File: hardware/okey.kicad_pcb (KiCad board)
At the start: 2 copper layers, 263.4 x 349.9 mm, 160 parts, among them IC1 4094N, IC2 4094N, J1 RJ45, J2 RJ45, P1 ROW_JMP, P10 CONN_02X06, P11 CONN_02X06, P12 CONN_02X06, P13 CONN_02X06, P14 CONN_02X06, P15 CONN_02X06, P16 CONN_02X08, P17 CONN_01X01, P18 CONN_02X08, P19 CONN_01X01, P2 CONN_02X13, P20 CONN_01X01, P21 CONN_01X01, P22 CONN_02X08, P23 CONN_02X08, P24 CONN_02X06, P25 CONN_02X06, P26 CONN_02X06, P27 CONN_02X06, P28 CONN_02X06, P29 CONN_02X06, P3 CONN_02X03, P30 CONN_02X08, P31 CONN_02X03, P32 CONN_02X03, P33 CONN_02X06, P34 CONN_02X06, P35 CONN_02X06, P36 CONN_02X06, P37 CONN_02X06, P38 CONN_02X06, P39 CONN_01X01, P4 CONN_02X08, P40 CONN_02X03, P41 CONN_02X06, P42 CONN_02X06, P43 CONN_02X06, P44 CONN_02X06, P45 CONN_02X06, P46 CONN_02X06, P47 CONN_01X01, P48 CONN_02X03, P5 CONN_02X03, P6 CONN_02X10, P7 CONN_02X03, P8 CONN_01X01, P9 CONN_02X08, Q1 Q_NPN_BCE, Q2 Q_NPN_BCE, Q3 Q_NPN_BCE, SW1 MX_D, SW10 MX_D, SW11 MX_D, SW12 MX_D, SW13 MX_D, SW14 MX_D, SW15 MX_D, SW16 MX_D, SW17 MX_D, SW18 MX_D, SW19 SW_PUSH, SW2 MX_D, SW20 SW_PUSH, SW21 SW_PUSH, SW22 SW_PUSH, SW23 SW_PUSH, SW24 SW_PUSH, SW25 SW_PUSH, SW26 SW_PUSH, SW27 SW_PUSH, SW28 SW_PUSH, SW29 SW_PUSH, SW3 MX_D, SW30 SW_PUSH, SW31 SW_PUSH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

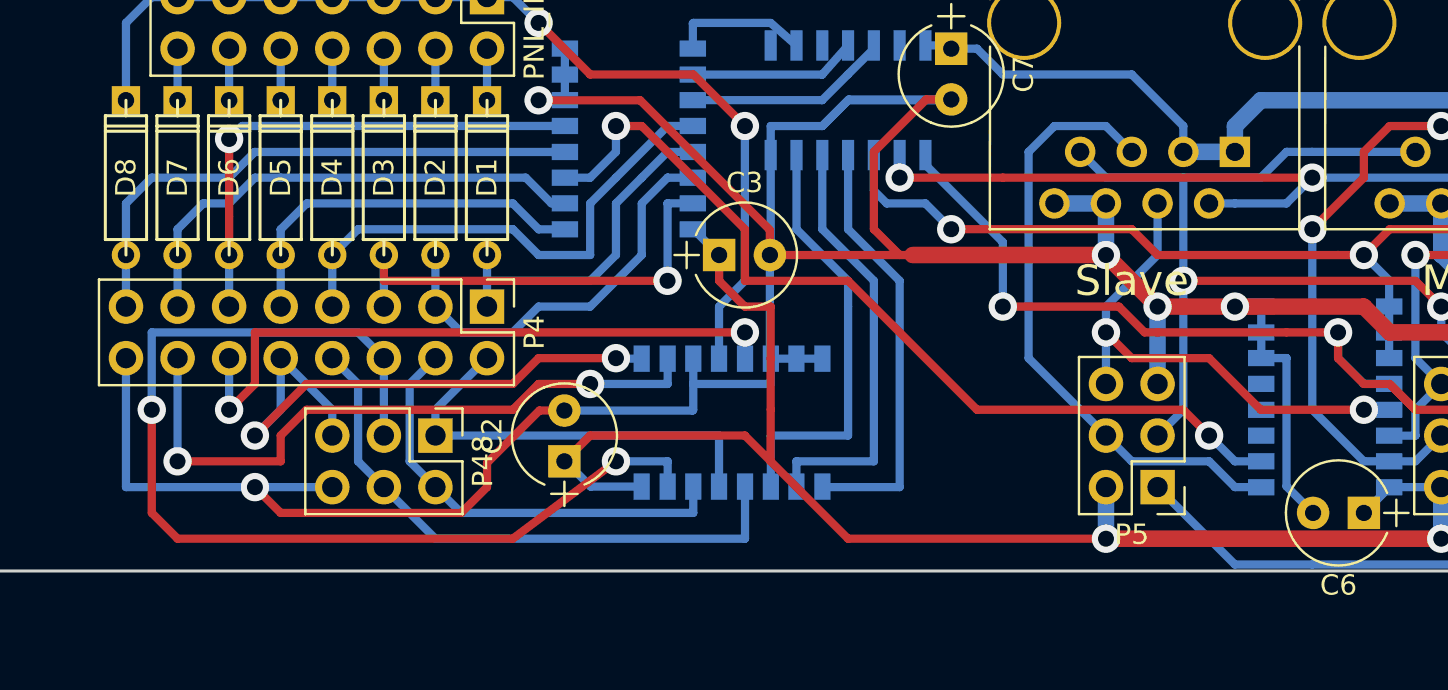
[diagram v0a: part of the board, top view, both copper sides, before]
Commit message: ...
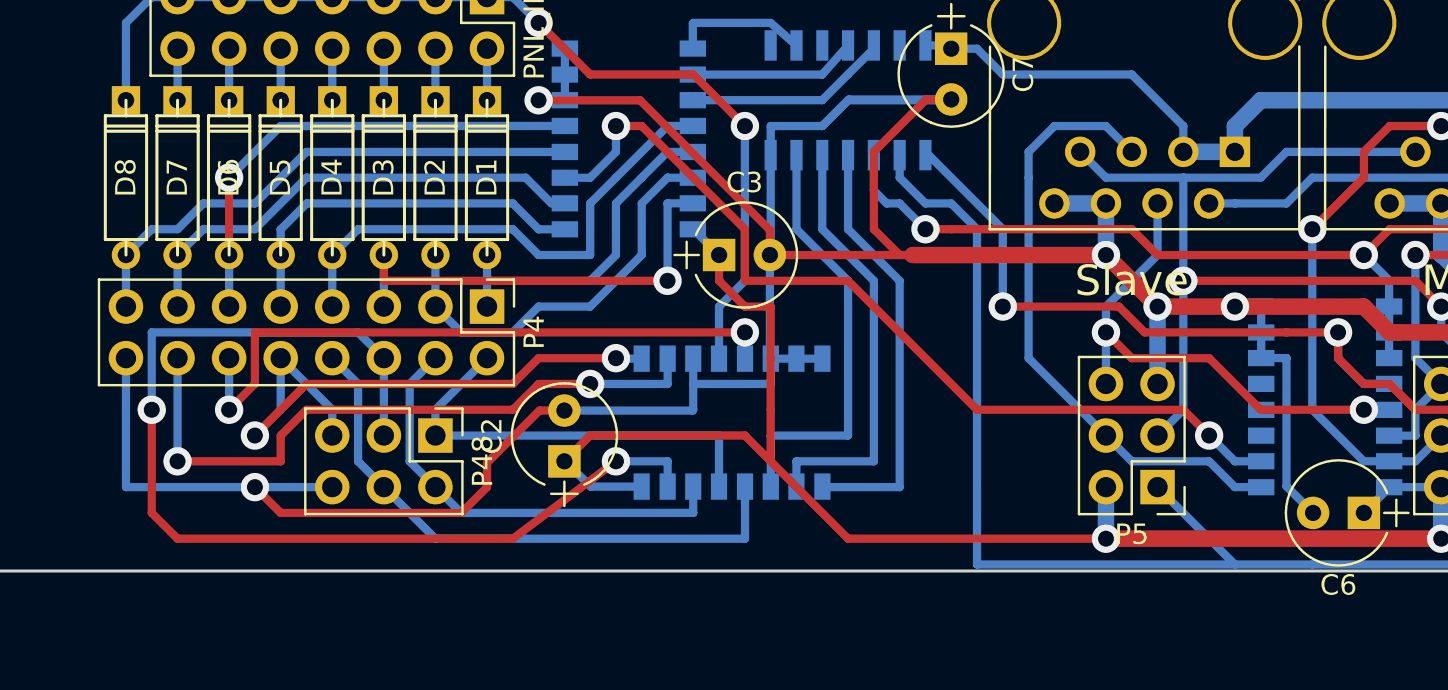
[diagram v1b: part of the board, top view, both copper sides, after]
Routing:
- net /Panel Generic SPI01/reset: track 85.6 -> 99.4 mm, vias 2 -> 0
- net Net-(D8-Pad2): track 27.7 -> 26.3 mm
- net Net-(D6-Pad2): track 25.1 -> 23.9 mm
- net Net-(D7-Pad2): track 24.5 -> 23.7 mm
- net Net-(IC1-Pad3): track 99.6 -> 100.2 mm
